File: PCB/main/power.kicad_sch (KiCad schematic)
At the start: 20 parts

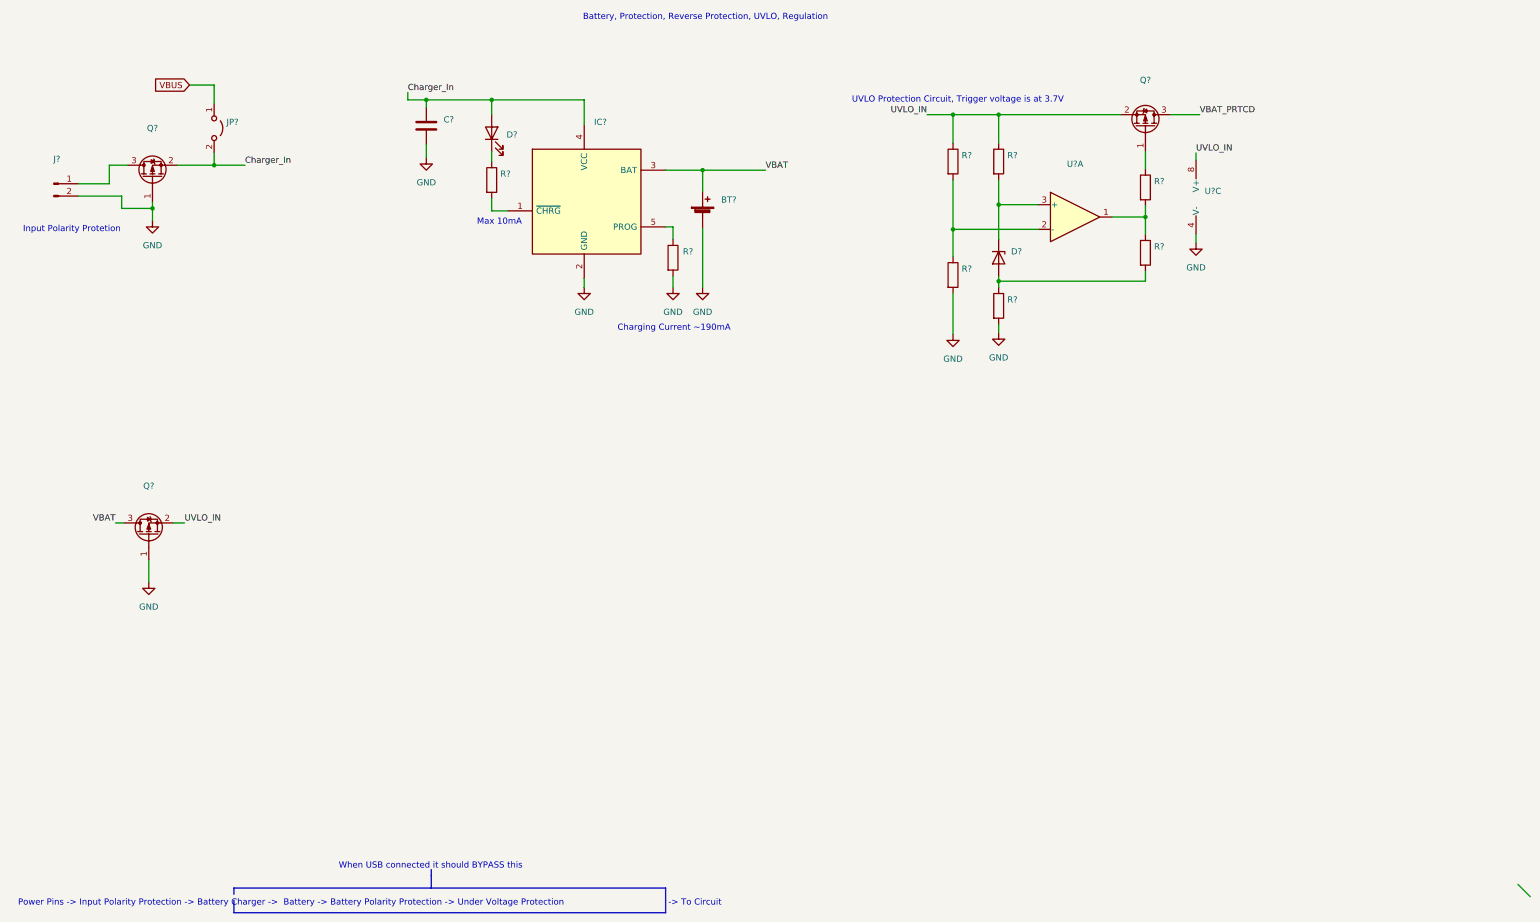
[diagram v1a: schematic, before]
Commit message: added eeprom and some usb-uart connections
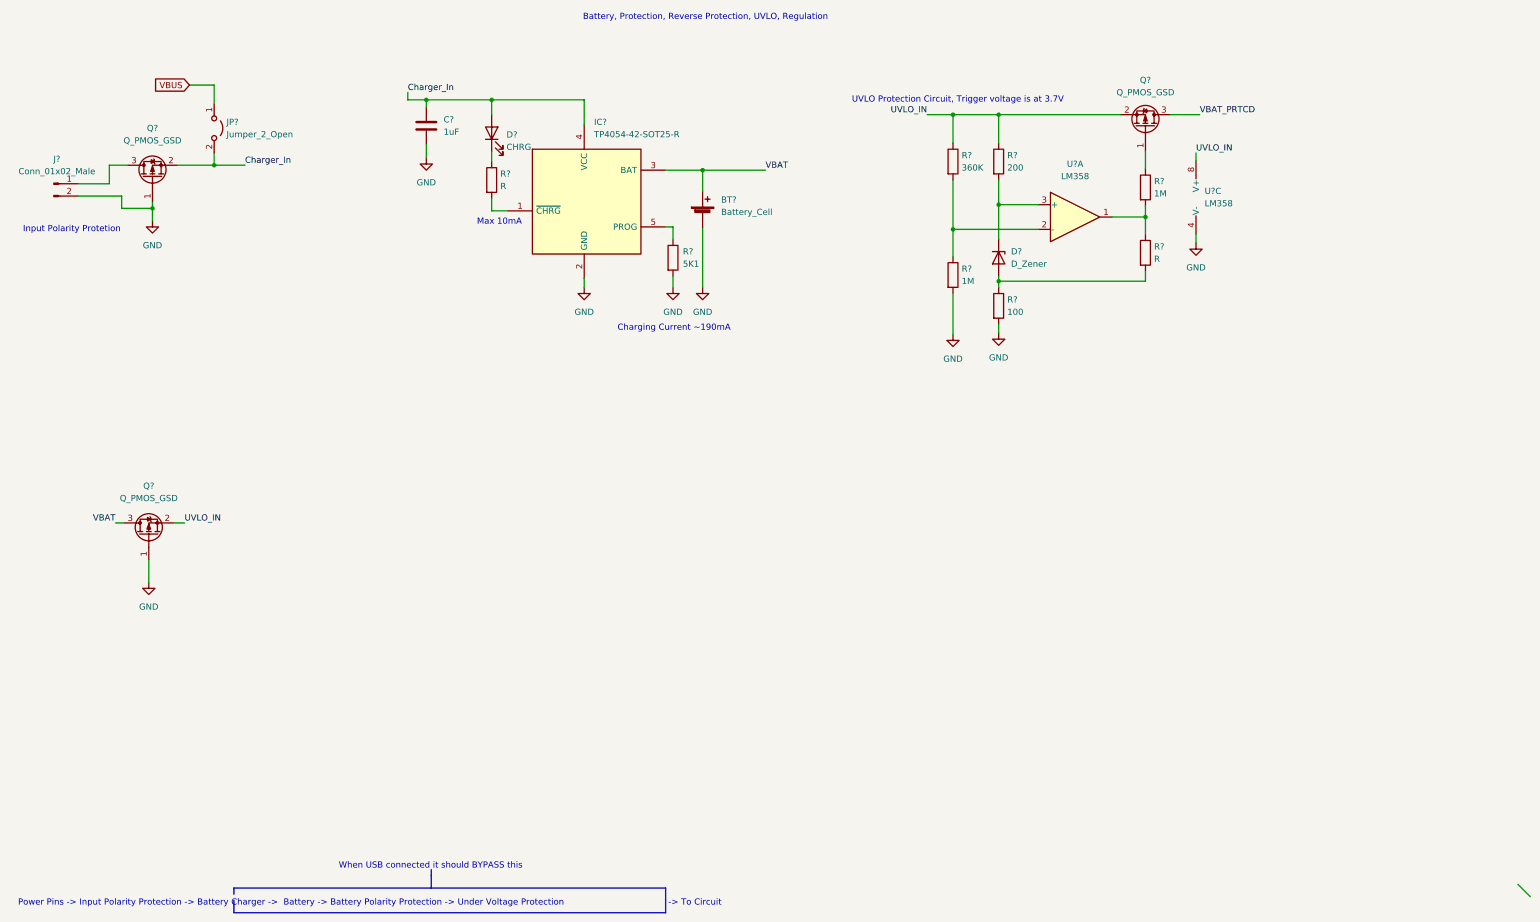
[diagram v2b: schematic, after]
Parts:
- BT?: value (none) -> Battery_Cell; footprint (none) -> Battery:BatteryHolder_Keystone_1042_1x18650
- C?: value (none) -> 1uF
- D?: value (none) -> D_Zener; footprint (none) -> Diode_SMD:D_SOD-523
- D?: value (none) -> CHRG
- IC?: value (none) -> TP4054-42-SOT25-R; footprint (none) -> SOT95P280X100-5N
- J?: value (none) -> Conn_01x02_Male
- JP?: value (none) -> Jumper_2_Open
- Q? (x3): value (none) -> Q_PMOS_GSD
- R? (x2): value (none) -> 1M; footprint (none) -> Resistor_SMD:R_0603_1608Metric_Pad0.98x0.95mm_HandSolder
- R?: value (none) -> 5K1; footprint (none) -> Resistor_SMD:R_0805_2012Metric_Pad1.20x1.40mm_HandSolder
- R?: value (none) -> 360K; footprint (none) -> Resistor_SMD:R_0603_1608Metric_Pad0.98x0.95mm_HandSolder
- R?: value (none) -> 200; footprint (none) -> Resistor_SMD:R_0603_1608Metric_Pad0.98x0.95mm_HandSolder
- R? (x2): value (none) -> R
- R?: value (none) -> 100; footprint (none) -> Resistor_SMD:R_0603_1608Metric_Pad0.98x0.95mm_HandSolder
- U?: value (none) -> LM358
- U?: value (none) -> LM358; footprint (none) -> Package_SO:SOIC-8_3.9x4.9mm_P1.27mm
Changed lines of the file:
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@@
     (in_bom yes) (on_board yes) (fields_autoplaced)
     (property "Reference" "Q?" (id 0) (at 252.476 20.32 90))
-    (property "Value" "" (id 1) (at 252.476 22.86 90))
+    (property "Value" "Q_PMOS_GSD" (id 1) (at 252.476 22.86 90))
     (property "Footprint" "" (id 2) (at 255.016 24.892 0)
       (effects (font (size 1.27 1.27)) hide)
@@
       (effects (font (size 1.27 1.27)) (justify left))
     )
-    (property "Value" "" (id 1) (at 214.63 61.7219 0)
-      (effects (font (size 1.27 1.27)) (justify left))
-    )
-    (property "Footprint" "" (id 2) (at 211.074 60.452 90)
+    (property "Value" "1M" (id 1) (at 214.63 61.7219 0)
+      (effects (font (size 1.27 1.27)) (justify left))
+    )
+    (property "Footprint" "Resistor_SMD:R_0603_1608Metric_Pad0.98x0.95mm_HandSolder" (id 2) (at 211.074 60.452 90)
       (effects (font (size 1.27 1.27)) hide)
     )
@@
       (effects (font (size 1.27 1.27)) (justify left))
     )
-    (property "Value" "" (id 1) (at 224.79 58.1659 90)
-      (effects (font (size 1.27 1.27)) (justify left))
-    )
-    (property "Footprint" "" (id 2) (at 222.25 56.896 0)
+    (property "Value" "D_Zener" (id 1) (at 224.79 58.1659 90)
+      (effects (font (size 1.27 1.27)) (justify left))
+    )
+    (property "Footprint" "Diode_SMD:D_SOD-523" (id 2) (at 222.25 56.896 0)
       (effects (font (size 1.27 1.27)) hide)
     )
@@
       (effects (font (size 1.27 1.27)) (justify left))
     )
-    (property "Value" "" (id 1) (at 157.226 58.1659 0)
-      (effects (font (size 1.27 1.27)) (justify left))
-    )
-    (property "Footprint" "" (id 2) (at 153.416 56.896 90)
+    (property "Value" "5K1" (id 1) (at 157.226 58.1659 0)
+      (effects (font (size 1.27 1.27)) (justify left))
+    )
+    (property "Footprint" "Resistor_SMD:R_0805_2012Metric_Pad1.20x1.40mm_HandSolder" (id 2) (at 153.416 56.896 90)
       (effects (font (size 1.27 1.27)) hide)
     )
@@
       (effects (font (size 1.27 1.27)) (justify left))
     )
-    (property "Value" "" (id 1) (at 214.63 38.3539 0)
-      (effects (font (size 1.27 1.27)) (justify left))
-    )
-    (property "Footprint" "" (id 2) (at 211.074 37.084 90)
+    (property "Value" "360K" (id 1) (at 214.63 38.3539 0)
+      (effects (font (size 1.27 1.27)) (justify left))
+    )
+    (property "Footprint" "Resistor_SMD:R_0603_1608Metric_Pad0.98x0.95mm_HandSolder" (id 2) (at 211.074 37.084 90)
       (effects (font (size 1.27 1.27)) hide)
     )
@@
       (effects (font (size 1.27 1.27)) (justify left))
     )
-    (property "Value" "" (id 1) (at 264.668 45.7199 0)
+    (property "Value" "LM358" (id 1) (at 264.668 45.7199 0)
       (effects (font (size 1.27 1.27)) (justify left))
     )
@@
       (effects (font (size 1.27 1.27)) (justify left))
     )
-    (property "Value" "" (id 1) (at 138.9254 31.496 0)
-      (effects (font (size 1.27 1.27)) (justify left))
-    )
-    (property "Footprint" "" (id 2) (at 163.83 42.672 0)
+    (property "Value" "TP4054-42-SOT25-R" (id 1) (at 138.9254 31.496 0)
+      (effects (font (size 1.27 1.27)) (justify left))
+    )
+    (property "Footprint" "SOT95P280X100-5N" (id 2) (at 163.83 42.672 0)
       (effects (font (size 1.27 1.27)) (justify left) hide)
     )
@@
     (in_bom yes) (on_board yes) (fields_autoplaced)
     (property "Reference" "U?" (id 0) (at 237.998 37.592 0))
-    (property "Value" "" (id 1) (at 237.998 40.132 0))
-    (property "Footprint" "" (id 2) (at 237.998 48.514 0)
+    (property "Value" "LM358" (id 1) (at 237.998 40.132 0))
+    (property "Footprint" "Package_SO:SOIC-8_3.9x4.9mm_P1.27mm" (id 2) (at 237.998 48.514 0)
       (effects (font (size 1.27 1.27)) hide)
     )
@@
     (in_bom yes) (on_board yes) (fields_autoplaced)
     (property "Reference" "J?" (id 0) (at 28.321 36.576 0))
-    (property "Value" "" (id 1) (at 28.321 39.116 0))
+    (property "Value" "Conn_01x02_Male" (id 1) (at 28.321 39.116 0))
     (property "Footprint" "" (id 2) (at 27.686 41.656 0)
       (effects (font (size 1.27 1.27)) hide)
@@
       (effects (font (size 1.27 1.27)) (justify left))
     )
-    (property "Value" "" (id 1) (at 224.028 38.3539 0)
-      (effects (font (size 1.27 1.27)) (justify left))
-    )
-    (property "Footprint" "" (id 2) (at 220.472 37.084 90)
+    (property "Value" "200" (id 1) (at 224.028 38.3539 0)
+      (effects (font (size 1.27 1.27)) (justify left))
+    )
+    (property "Footprint" "Resistor_SMD:R_0603_1608Metric_Pad0.98x0.95mm_HandSolder" (id 2) (at 220.472 37.084 90)
       (effects (font (size 1.27 1.27)) hide)
     )
@@
       (effects (font (size 1.27 1.27)) (justify left))
     )
-    (property "Value" "" (id 1) (at 254.254 57.1499 0)
+    (property "Value" "R" (id 1) (at 254.254 57.1499 0)
       (effects (font (size 1.27 1.27)) (justify left))
     )
@@
       (effects (font (size 1.27 1.27)) (justify left))
     )
-    (property "Value" "" (id 1) (at 254.254 43.6879 0)
-      (effects (font (size 1.27 1.27)) (justify left))
-    )
-    (property "Footprint" "" (id 2) (at 250.698 42.418 90)
+    (property "Value" "1M" (id 1) (at 254.254 43.6879 0)
+      (effects (font (size 1.27 1.27)) (justify left))
+    )
+    (property "Footprint" "Resistor_SMD:R_0603_1608Metric_Pad0.98x0.95mm_HandSolder" (id 2) (at 250.698 42.418 90)
       (effects (font (size 1.27 1.27)) hide)
     )
@@
       (effects (font (size 1.27 1.27)) (justify right))
     )
-    (property "Value" "" (id 1) (at 120.904 34.0994 90)
+    (property "Value" "CHRG" (id 1) (at 120.904 34.0994 90)
       (effects (font (size 1.27 1.27)) (justify right))
     )
@@
       (effects (font (size 1.27 1.27)) (justify left))
     )
-    (property "Value" "" (id 1) (at 63.246 31.4959 90)
+    (property "Value" "Jumper_2_Open" (id 1) (at 63.246 31.4959 90)
       (effects (font (size 1.27 1.27)) (justify left))
     )
@@
     (in_bom yes) (on_board yes) (fields_autoplaced)
     (property "Reference" "Q?" (id 0) (at 48.006 30.226 90))
-    (property "Value" "" (id 1) (at 48.006 32.766 90))
+    (property "Value" "Q_PMOS_GSD" (id 1) (at 48.006 32.766 90))
     (property "Footprint" "" (id 2) (at 45.466 35.306 0)
       (effects (font (size 1.27 1.27)) hide)
@@
       (effects (font (size 1.27 1.27)) (justify left))
     )
-    (property "Value" "" (id 1) (at 119.634 42.1639 0)
+    (property "Value" "R" (id 1) (at 119.634 42.1639 0)
       (effects (font (size 1.27 1.27)) (justify left))
     )
@@
       (effects (font (size 1.27 1.27)) (justify left))
     )
-    (property "Value" "" (id 1) (at 165.1 47.4979 0)
-      (effects (font (size 1.27 1.27)) (justify left))
-    )
-    (property "Footprint" "" (id 2) (at 161.29 46.736 90)
+    (property "Value" "Battery_Cell" (id 1) (at 165.1 47.4979 0)
+      (effects (font (size 1.27 1.27)) (justify left))
+    )
+    (property "Footprint" "Battery:BatteryHolder_Keystone_1042_1x18650" (id 2) (at 161.29 46.736 90)
       (effects (font (size 1.27 1.27)) hide)
     )
@@
     (in_bom yes) (on_board yes) (fields_autoplaced)
     (property "Reference" "Q?" (id 0) (at 47.244 103.886 90))
-    (property "Value" "" (id 1) (at 47.244 106.426 90))
+    (property "Value" "Q_PMOS_GSD" (id 1) (at 47.244 106.426 90))
     (property "Footprint" "" (id 2) (at 44.704 108.966 0)
       (effects (font (size 1.27 1.27)) hide)
@@
       (effects (font (size 1.27 1.27)) (justify left))
     )
-    (property "Value" "" (id 1) (at 107.95 30.9879 0)
+    (property "Value" "1uF" (id 1) (at 107.95 30.9879 0)
       (effects (font (size 1.27 1.27)) (justify left))
     )
@@
       (effects (font (size 1.27 1.27)) (justify left))
     )
-    (property "Value" "" (id 1) (at 224.028 68.0719 0)
-      (effects (font (size 1.27 1.27)) (justify left))
-    )
-    (property "Footprint" "" (id 2) (at 220.472 66.802 90)
-      (effects (font (size 1.27 1.27)) hide)
-    )
+    (property "Value" "100" (id 1) (at 224.028 68.0719 0)
+      (effects (font (size 1.27 1.27)) (justify left))
+    )
+    (property "Footprint" "Resistor_SMD:R_0603_1608Metric_Pad0.98x0.95mm_HandSolder" (id 2) (at 220.472 66.802 90)
+      (effects (font (size 1.27 1.27)) hide)
+    )
